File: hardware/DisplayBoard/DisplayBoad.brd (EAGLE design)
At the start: 100 x 54.6 mm, 45 parts, among them IC1 MCP23017, SW1 EC12E_SW, SW2 EC12E_SW, U1 EADOGL128-6

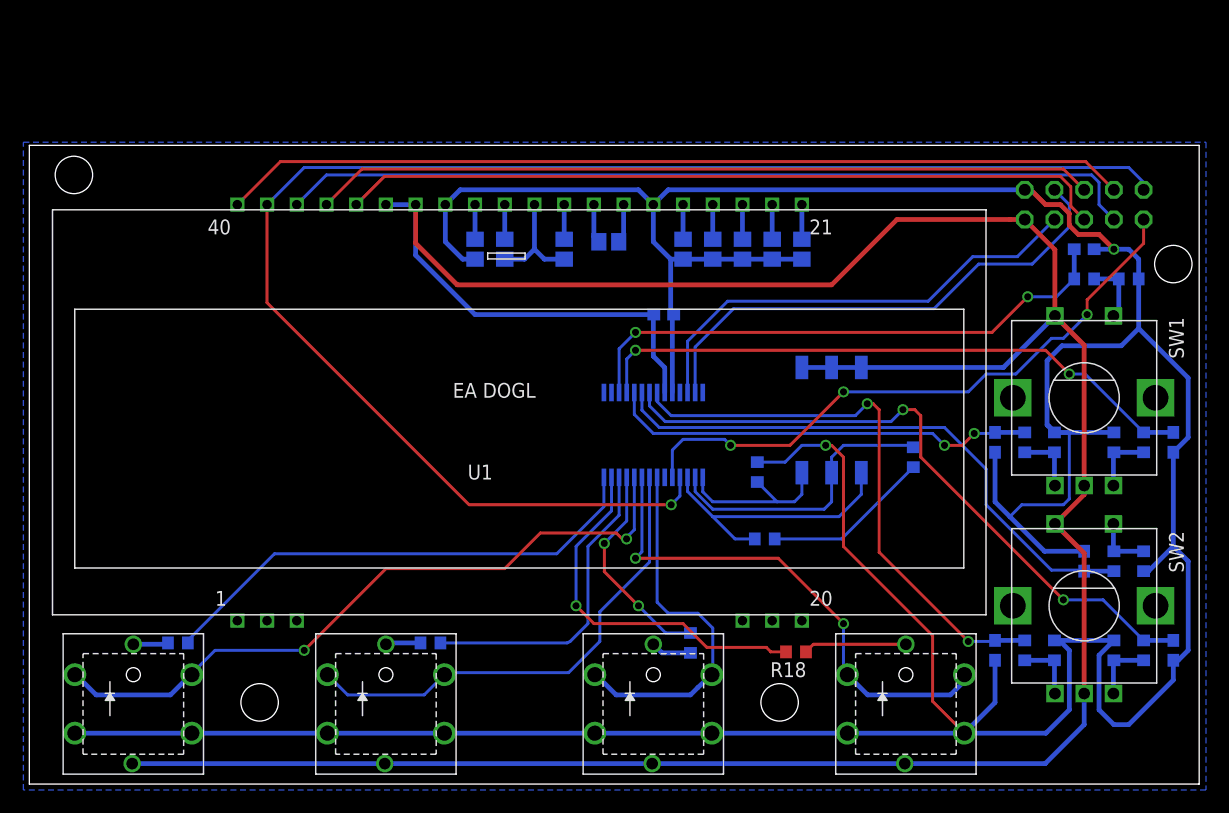
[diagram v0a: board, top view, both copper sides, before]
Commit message: Updates
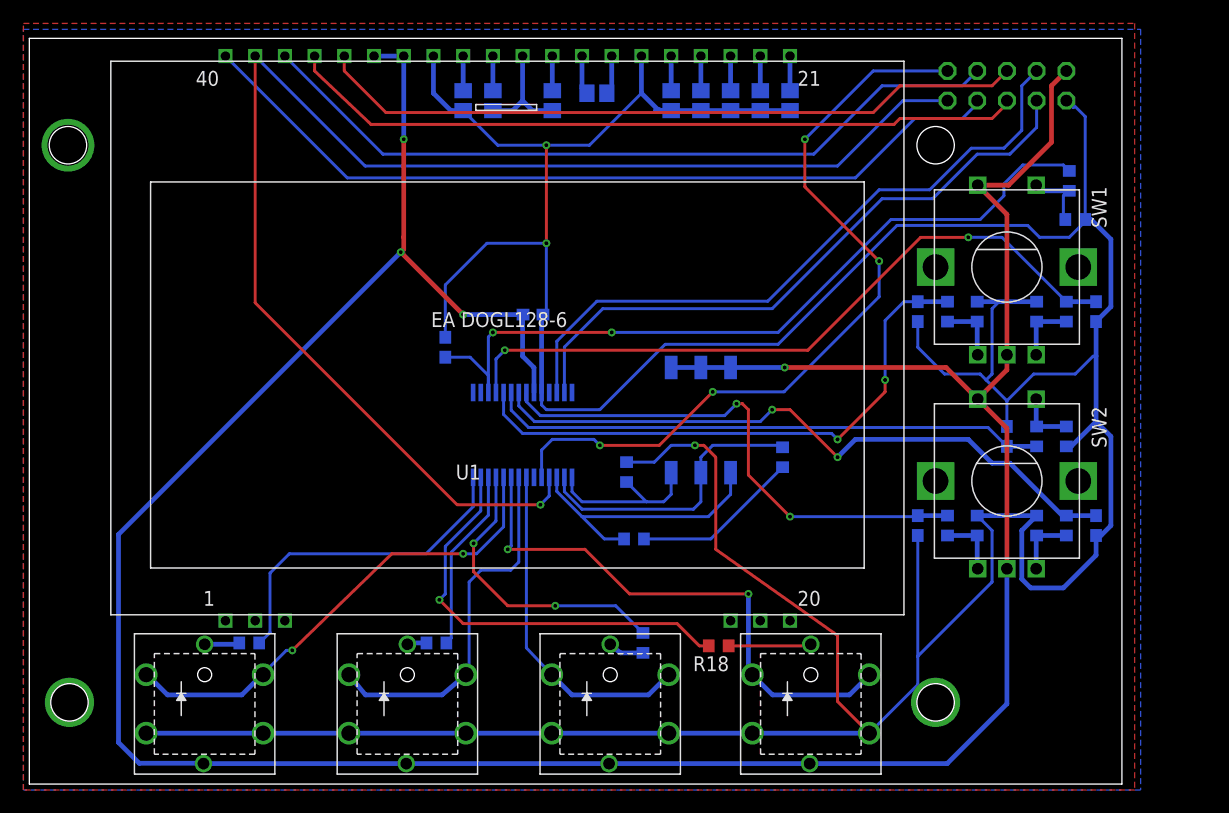
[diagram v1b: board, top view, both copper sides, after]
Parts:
- U1: value EADOGL128-6 -> EADOGL128-62; device ea:EADOGL -> ea:EA_DOGL128-6
- moved C12 55.2 mm to (35.6, 37.3), turned to 270 degrees
- moved C10 13.0 mm to (75.9, 40.4)
- moved C11 13.0 mm to (91.2, 40.4)
- moved R2 13.0 mm to (88.6, 40.4)
- moved R3 13.0 mm to (78.5, 40.4)
- moved R5 13.0 mm to (86.1, 40.4)
- moved R6 13.0 mm to (81.0, 40.4)
- moved SW1 13.0 mm to (83.6, 44.2)
- moved C1 12.7 mm to (37.1, 58.4)
- moved C2 12.7 mm to (54.9, 58.4)
- moved C3 12.7 mm to (57.4, 58.4)
- moved C4 12.7 mm to (59.9, 58.4)
- moved C5 12.7 mm to (62.5, 58.4)
- moved C6 12.7 mm to (65.0, 58.4)
- moved C7 12.7 mm to (39.6, 58.4)
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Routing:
- net GND: track 361.0 -> 386.8 mm, vias 2 -> 6
- net ENC1_T: track 47.7 -> 67.2 mm
- net DISP_S3: track 59.6 -> 41.6 mm
- net I2C_SCL: track 40.1 -> 57.2 mm
- net INT: track 53.1 -> 67.7 mm, vias 3 -> 4
- net GPA7: track 43.0 -> 28.8 mm
- net ENC1_S2: track 36.8 -> 49.2 mm
- net GPA5: track 26.9 -> 15.6 mm
- net I2C_SDA: track 43.8 -> 54.3 mm
- net VCC: track 250.1 -> 260.3 mm, vias 0 -> 4
- net DISP_S1: track 41.7 -> 31.6 mm
- net RESET: track 130.1 -> 120.7 mm
- net MODE: track 73.6 -> 65.6 mm
- net ENC1_S1: track 52.8 -> 60.7 mm
- net GPA4: track 18.4 -> 25.5 mm
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- added copper zone on layer 1, net GND
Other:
- board size 100 x 54.6 mm -> 93.4 x 63.7 mm
- board text added: "05/2013"
- board text added: "peschuster.de"
